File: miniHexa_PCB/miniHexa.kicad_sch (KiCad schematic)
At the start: 22 parts, among them SW1 SW_Push, U1 STM32F401RETx, Y2 25mhz

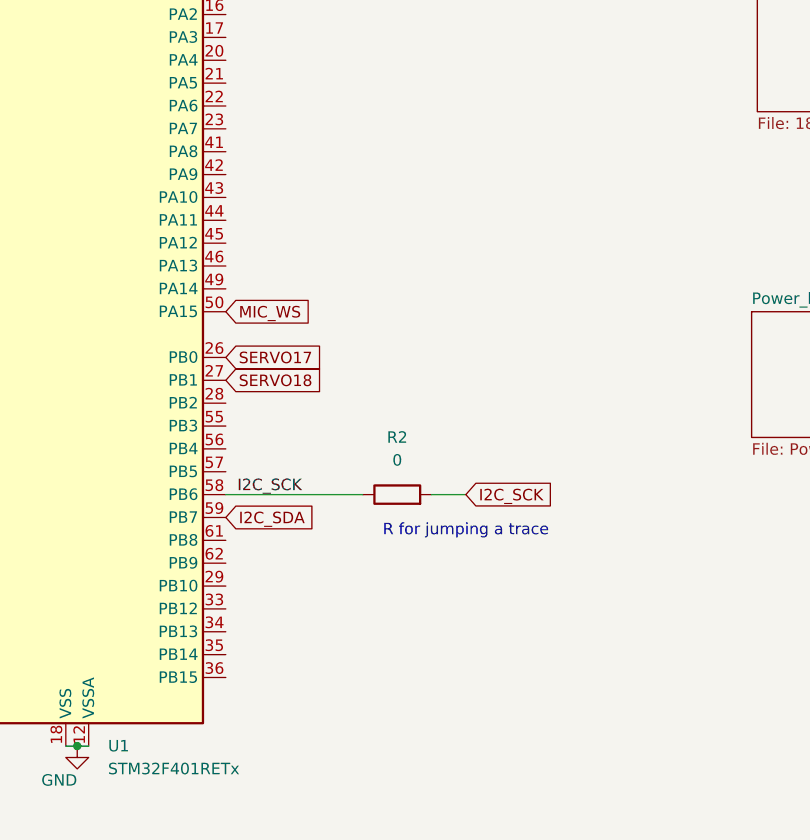
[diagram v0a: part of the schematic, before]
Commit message: start of version 2.0
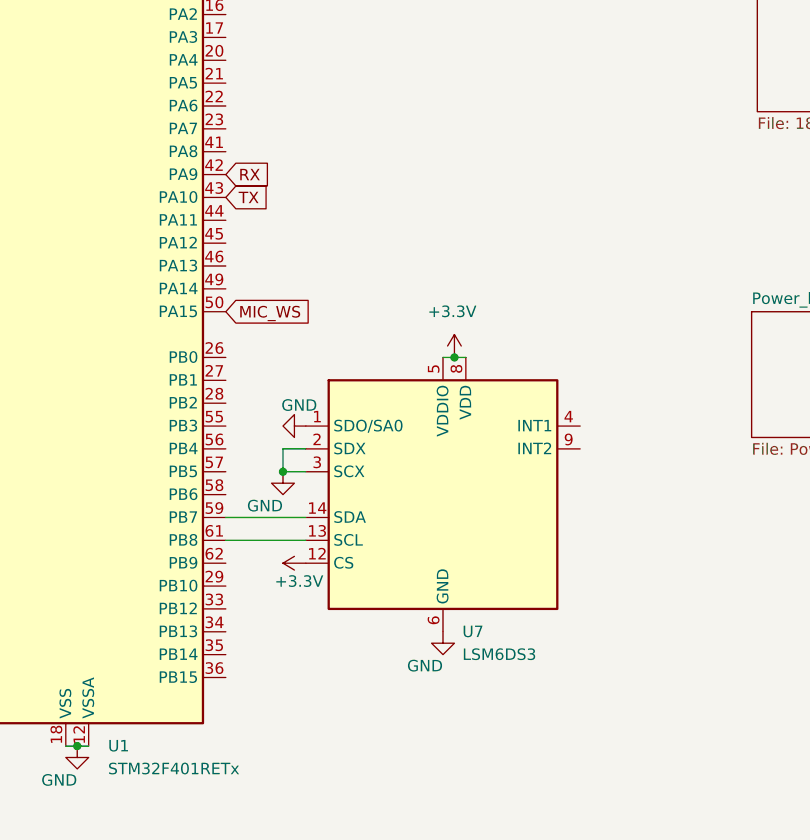
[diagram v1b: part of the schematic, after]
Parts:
- removed R2: 0, Resistor_SMD:R_0603_1608Metric, symbol Device:R
- added U7: LSM6DS3, Package_LGA:LGA-14_3x2.5mm_P0.5mm_LayoutBorder3x4y, symbol Sensor_Motion:LSM6DS3
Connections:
- net +3.3V: now also U7.12 (CS), U7.5 (VDDIO), U7.8 (VDD)
- net GND: now also U7.1 (SDO/SA0), U7.2 (SDX), U7.3 (SCX), U7.6 (GND), U7.7 (GND)
- net RX: now reaches U1.42 (PA9)
- net TX: now reaches U1.43 (PA10)
- net at U1.61 (PB8): now also U7.13 (SCL)
- net I2C_SCK: no longer names the net of U1.58 (PB6)
- net I2C_SDA: no longer names the net of U1.59 (PB7)
- net I2C_SDA: now also U7.14 (SDA)
- net SERVO17: no longer names the net of U1.26 (PB0)
- net SERVO18: no longer names the net of U1.27 (PB1)
